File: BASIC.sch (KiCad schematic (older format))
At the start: 2 parts, among them U4 27C010

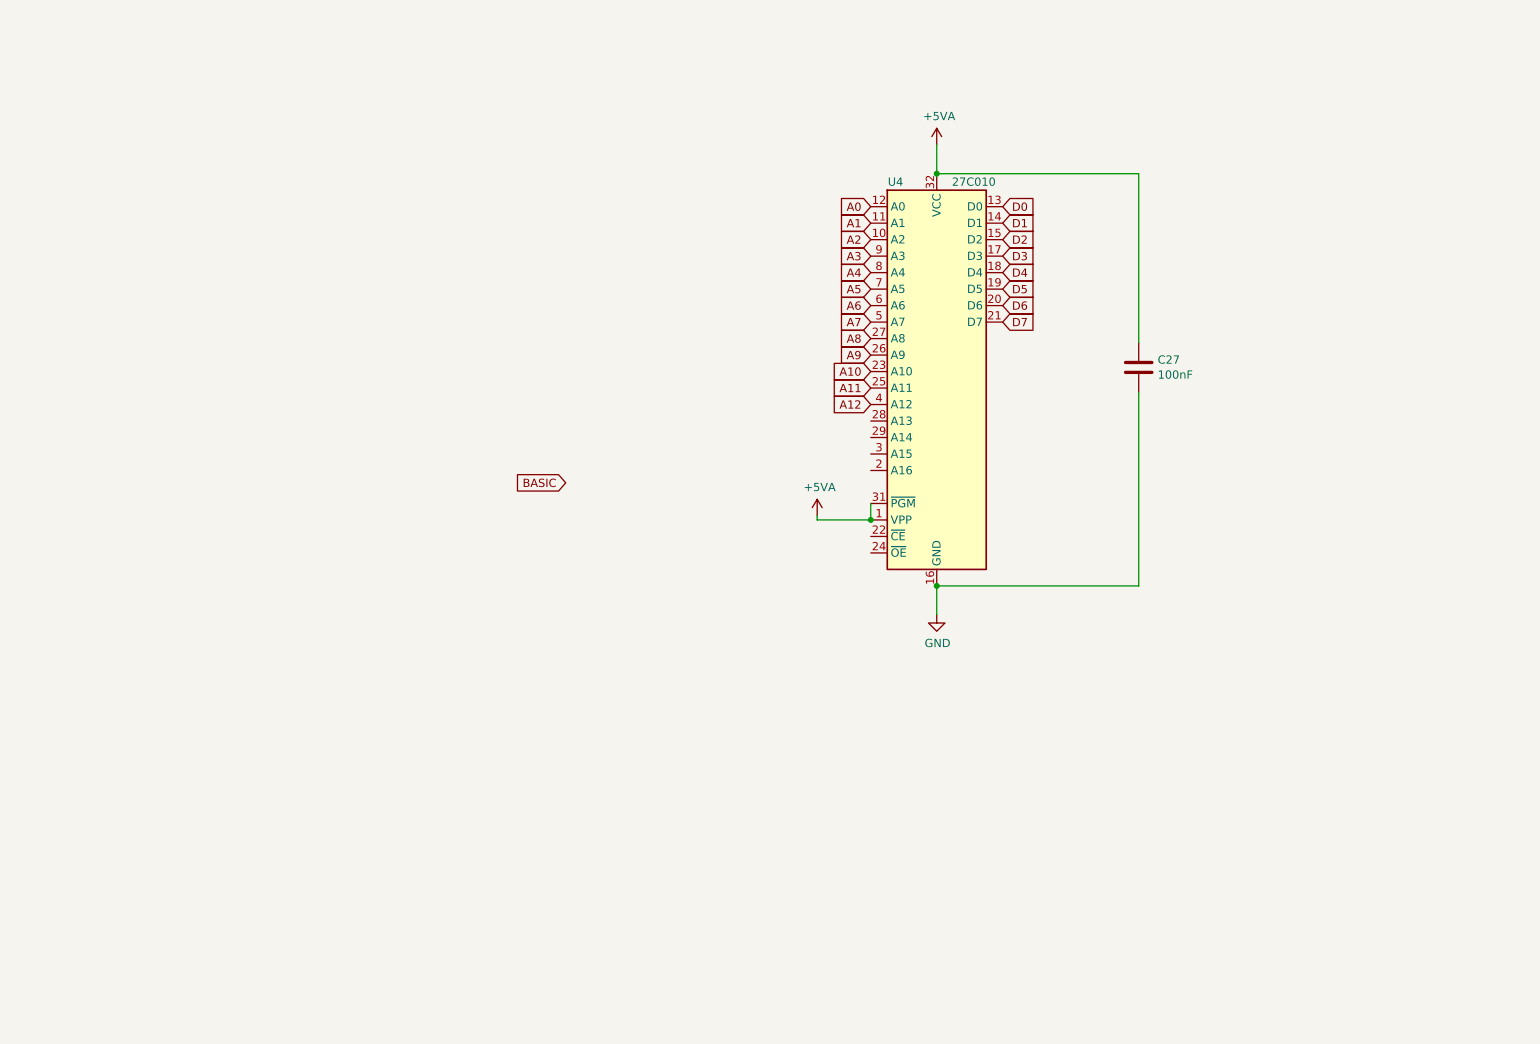
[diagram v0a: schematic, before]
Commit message: SuperCart
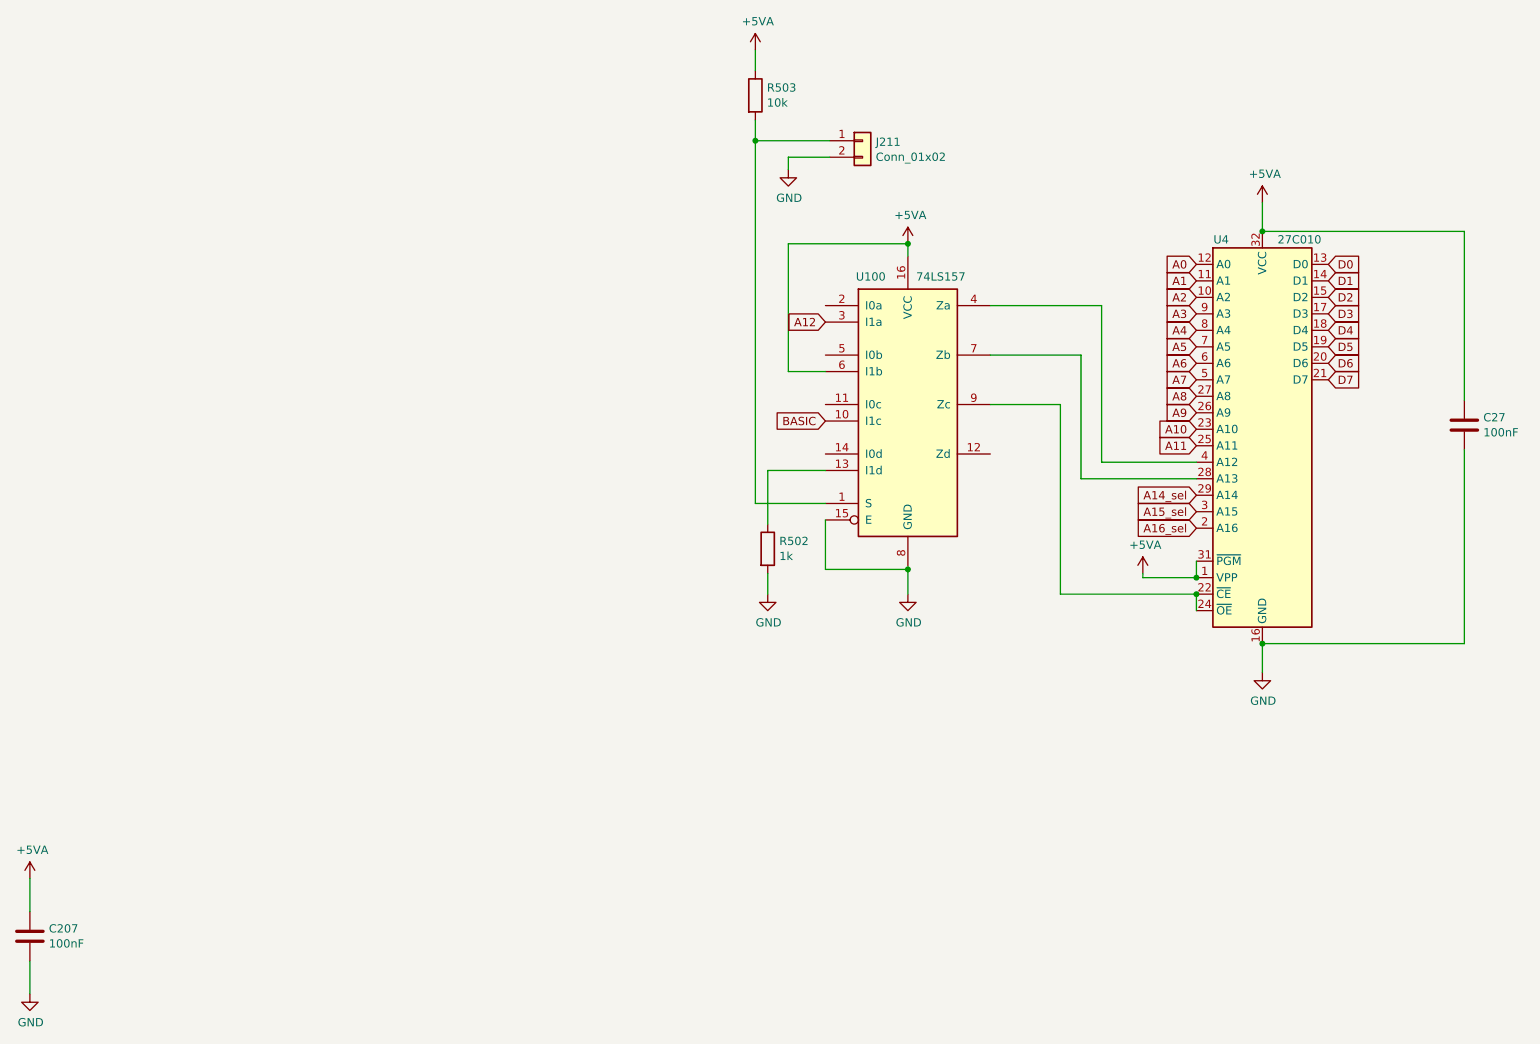
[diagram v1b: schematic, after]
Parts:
- added C207: 100nF, Capacitor_SMD:C_1206_3216Metric_Pad1.42x1.75mm_HandSolder, symbol Device:C
- added J211: Conn_01x02, Connector_PinHeader_2.54mm:PinHeader_1x02_P2.54mm_Vertical, symbol Connector_Generic:Conn_01x02
- added R502: 1k, Resistor_SMD:R_1206_3216Metric_Pad1.42x1.75mm_HandSolder, symbol Device:R
- added R503: 10k, Resistor_SMD:R_1206_3216Metric_Pad1.42x1.75mm_HandSolder, symbol Device:R
- added U100: 74LS157, Package_SO:SOIC-16_3.9x9.9mm_P1.27mm, symbol 74xx:74LS157
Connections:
- net +5VA: now also C207.1, R503.1, U100.16 (VCC), U100.6 (I1b)
- net A12: now also U100.3 (I1a); no longer U4.4 (A12)
- net BASIC: now also U100.10 (I1c)
- net GND: now also C207.2, J211.2 (Pin_2), R502.2, U100.15 (E), U100.8 (GND)
- net A16_sel: now reaches U4.2 (A16)
- net at U4.22 (~CE): now also U4.24 (~OE), U100.9 (Zc)
- net at U4.28 (A13): now also U100.7 (Zb)
- net A14_sel: now reaches U4.29 (A14)
- net A15_sel: now reaches U4.3 (A15)
- new net: U100.4 (Za), U4.4 (A12)
- new net: J211.1 (Pin_1), R503.2, U100.1 (S)
- new net: R502.1, U100.13 (I1d)
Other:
- moved on the sheet: C27, U4
